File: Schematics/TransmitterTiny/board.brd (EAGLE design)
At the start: 100 x 80 mm, 12 parts, among them IC1 TINY13-20PU, T1 2N2222

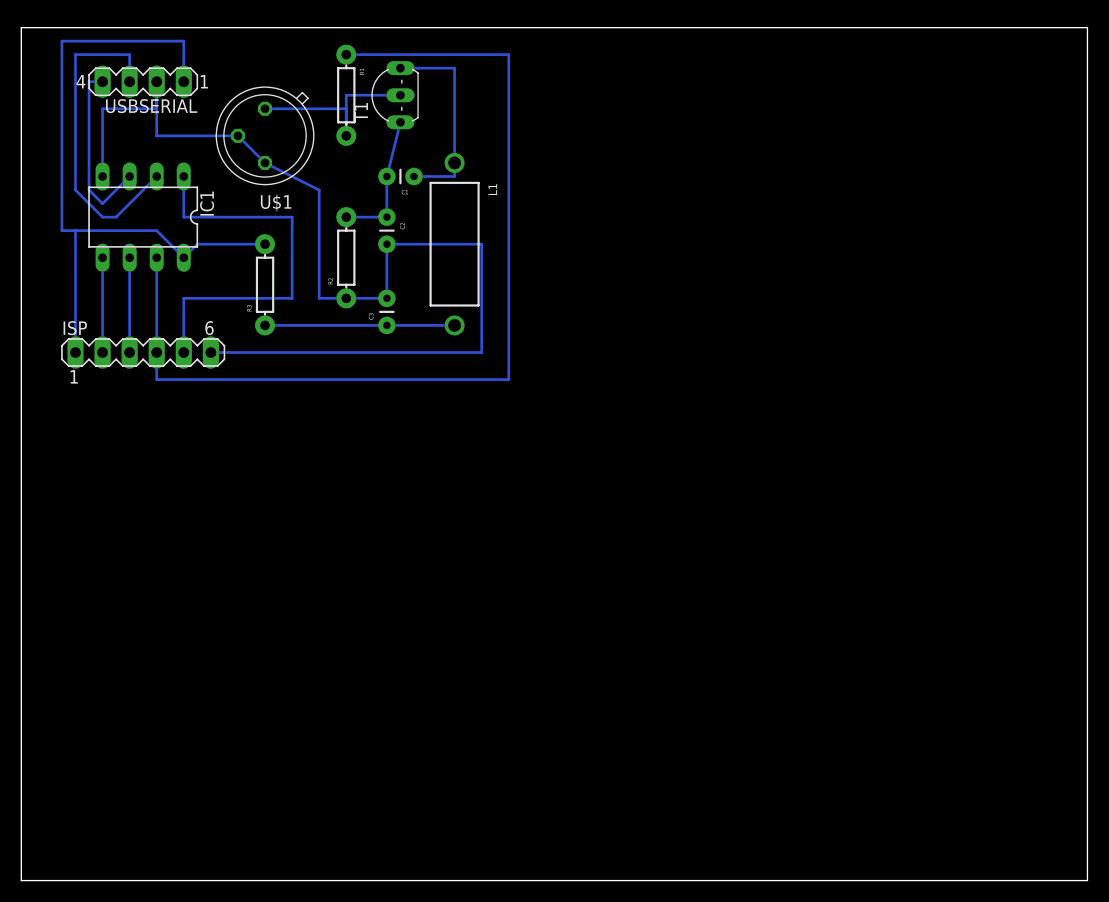
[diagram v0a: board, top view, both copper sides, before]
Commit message: Finished board
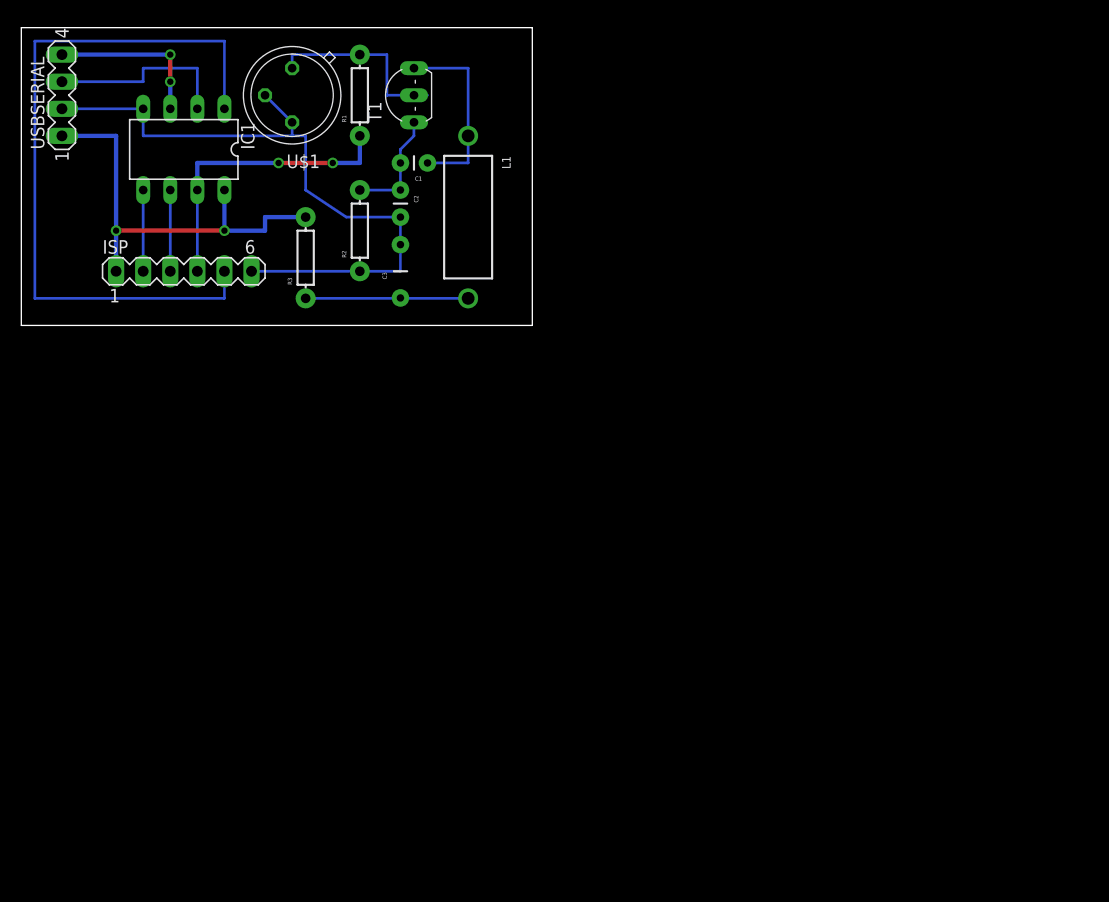
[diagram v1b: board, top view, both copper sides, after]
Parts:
- C3: device SparkFun-Capacitors:CAP-PTH-SMALL -> SparkFun-Capacitors:CAP-PTH-5MM
- moved ISP 8.52 mm to (15.2, 57.1)
- moved USBSERIAL 7.73 mm to (3.81, 73.7), turned to 90 degrees
- moved IC1 7.41 mm to (15.2, 68.6)
- moved C3 5.24 mm to (35.6, 57.1)
- moved R3 4.58 mm to (26.7, 58.4)
- moved U$1 4.58 mm to (25.4, 73.7)
- moved C2 2.84 mm to (35.6, 64.8)
- moved R2 2.84 mm to (31.8, 61.0)
- moved L1 2.84 mm to (41.9, 62.2)
- moved C1 1.80 mm to (38.1, 67.3)
- moved T1 1.27 mm to (35.6, 73.7)
- moved R1 1.27 mm to (31.8, 73.7), turned to 90 degrees
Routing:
- net N$5: track 90.2 -> 27.9 mm, vias 0 -> 2
- net N$8: track 102.0 -> 64.1 mm
- net N$12: track 36.8 -> 68.6 mm
- net N$2: track 65.1 -> 40.6 mm, vias 0 -> 2
- net N$3: track 30.6 -> 17.8 mm
- net N$6: track 20.3 -> 17.8 mm
- net N$7: track 17.8 -> 15.3 mm
- net N$9: track 12.9 -> 10.7 mm
- net N$4: track 16.8 -> 15.2 mm, vias 0 -> 2
- net N$15: track 8.89 -> 7.62 mm
- net N$14: track 8.89 -> 7.62 mm
- net N$11: track 19.0 -> 17.8 mm
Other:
- board size 100 x 80 mm -> 47.9 x 27.9 mm
